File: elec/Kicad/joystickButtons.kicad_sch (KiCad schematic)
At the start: 10 parts, among them SW1 SW_Push_Gauche_GO_IN, SW2 SW_Push_Droite_GO_BACK, SW3 SW_Push_Action_LOG_EXIT

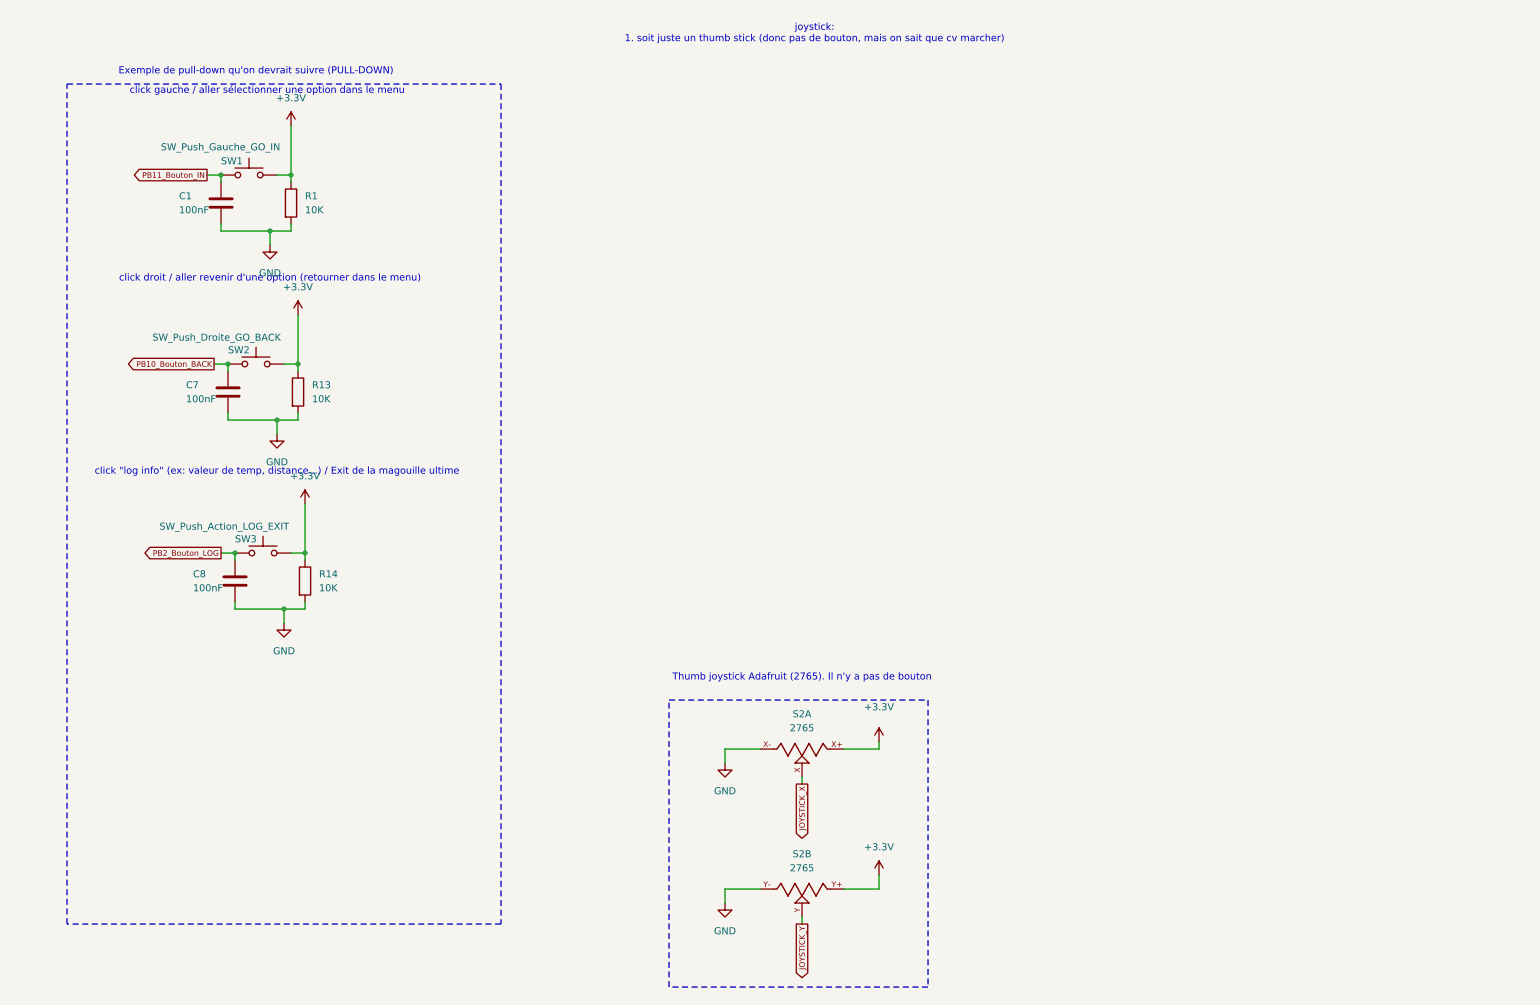
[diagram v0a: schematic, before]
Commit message: touillerie
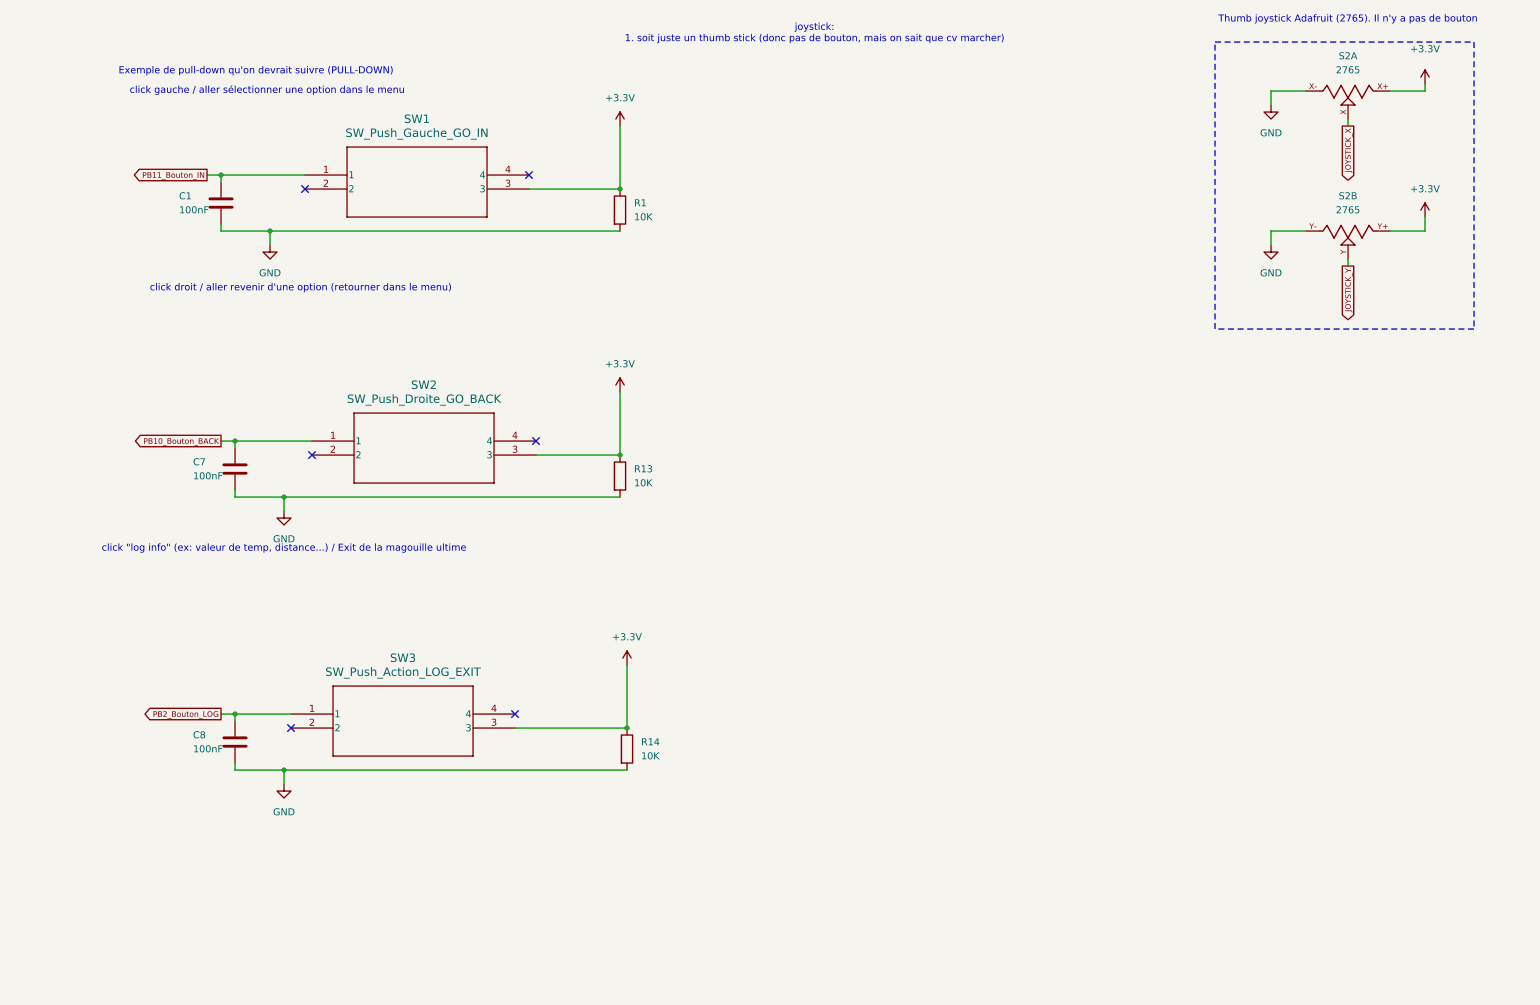
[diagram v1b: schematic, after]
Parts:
- removed SW1: SW_Push_Gauche_GO_IN, Button_Switch_SMD:SW_SPST_PTS645, symbol Switch:SW_Push
- removed SW2: SW_Push_Droite_GO_BACK, Button_Switch_SMD:SW_SPST_PTS645, symbol Switch:SW_Push
- removed SW3: SW_Push_Action_LOG_EXIT, Button_Switch_SMD:SW_SPST_PTS645, symbol Switch:SW_Push
- added SW1: SW_Push_Gauche_GO_IN, tacticleSwitch4_5x4_5mm:SWITCH_TR2LFS, symbol tacticleSwitch4_5x4_5mm:PTS647SN70SMTR2LFS
- added SW2: SW_Push_Droite_GO_BACK, tacticleSwitch4_5x4_5mm:SWITCH_TR2LFS, symbol tacticleSwitch4_5x4_5mm:PTS647SN70SMTR2LFS
- added SW3: SW_Push_Action_LOG_EXIT, tacticleSwitch4_5x4_5mm:SWITCH_TR2LFS, symbol tacticleSwitch4_5x4_5mm:PTS647SN70SMTR2LFS
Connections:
- net +3.3V: now also SW1.3, SW2.3, SW3.3
- net PB10_Bouton_BACK: now also SW2.1
- net PB11_Bouton_IN: now also SW1.1
- net PB2_Bouton_LOG: now also SW3.1
- no-connect marks 0 -> 6
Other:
- moved on the sheet: C7, C8, R1, R13, R14, S2A, S2B

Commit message: Jpense pas boire jeudi sérieux vue que y'a pas de 5@8
routage du découplage et des CLK
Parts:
- C1, C7, C8: footprint Capacitor_SMD:C_0603_1608Metric_Pad1.08x0.95mm_HandSolder -> Capacitor_SMD:C_0402_1005Metric_Pad0.74x0.62mm_HandSolder
- R1, R13, R14: footprint Resistor_SMD:R_0603_1608Metric_Pad0.98x0.95mm_HandSolder -> Resistor_SMD:R_0402_1005Metric_Pad0.72x0.64mm_HandSolder
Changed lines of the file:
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@@
 			)
 		)
-		(property "Footprint" "Resistor_SMD:R_0603_1608Metric_Pad0.98x0.95mm_HandSolder"
+		(property "Footprint" "Resistor_SMD:R_0402_1005Metric_Pad0.72x0.64mm_HandSolder"
 			(at 118.872 149.86 90)
 			(effects
@@
 			)
 		)
-		(property "Footprint" "Capacitor_SMD:C_0603_1608Metric_Pad1.08x0.95mm_HandSolder"
+		(property "Footprint" "Capacitor_SMD:C_0402_1005Metric_Pad0.74x0.62mm_HandSolder"
 			(at 50.4952 152.4 0)
 			(effects
@@
 			)
 		)
-		(property "Footprint" "Capacitor_SMD:C_0603_1608Metric_Pad1.08x0.95mm_HandSolder"
+		(property "Footprint" "Capacitor_SMD:C_0402_1005Metric_Pad0.74x0.62mm_HandSolder"
 			(at 50.4952 102.87 0)
 			(effects
@@
 			)
 		)
-		(property "Footprint" "Capacitor_SMD:C_0603_1608Metric_Pad1.08x0.95mm_HandSolder"
+		(property "Footprint" "Capacitor_SMD:C_0402_1005Metric_Pad0.74x0.62mm_HandSolder"
 			(at 47.9552 54.61 0)
 			(effects
@@
 			)
 		)
-		(property "Footprint" "Resistor_SMD:R_0603_1608Metric_Pad0.98x0.95mm_HandSolder"
+		(property "Footprint" "Resistor_SMD:R_0402_1005Metric_Pad0.72x0.64mm_HandSolder"
 			(at 117.602 52.07 90)
 			(effects
@@
 			)
 		)
-		(property "Footprint" "Resistor_SMD:R_0603_1608Metric_Pad0.98x0.95mm_HandSolder"
+		(property "Footprint" "Resistor_SMD:R_0402_1005Metric_Pad0.72x0.64mm_HandSolder"
 			(at 117.602 100.33 90)
 			(effects
